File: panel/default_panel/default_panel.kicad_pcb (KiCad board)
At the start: 2 copper layers, 100 x 100 mm, 1 part

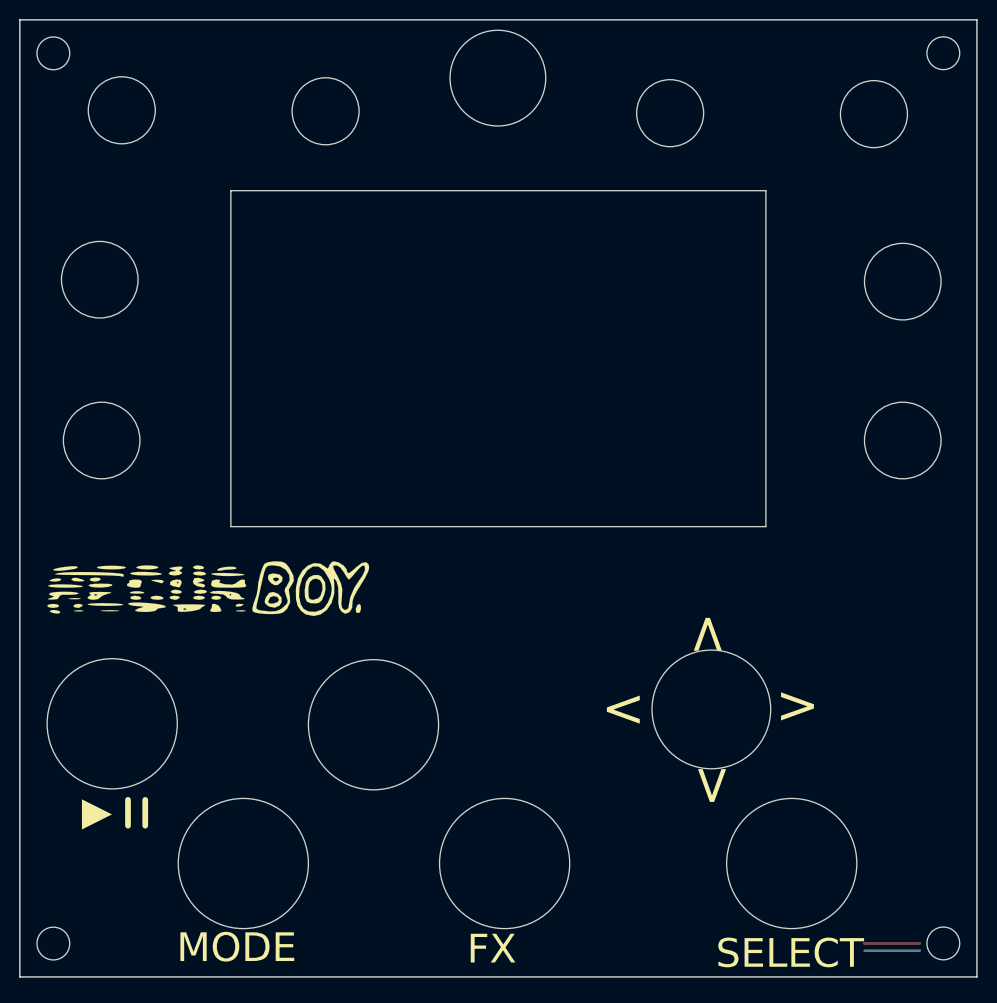
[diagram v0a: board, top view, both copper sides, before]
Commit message: add panel stuff
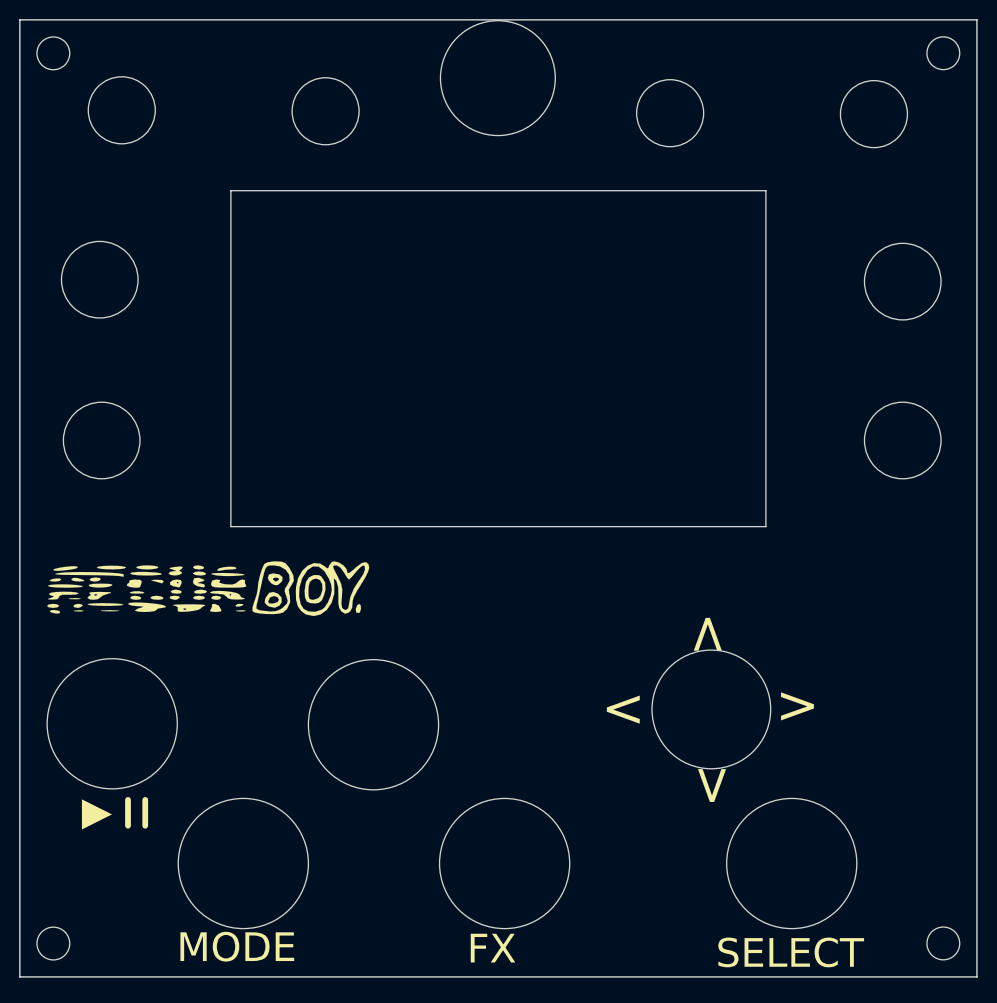
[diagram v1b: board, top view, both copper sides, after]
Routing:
- net (no net): track 11.6 -> 0.00 mm
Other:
- outline, holes or cut-outs redrawn
- board text added: "default_panel mk_iii for recurBOY v0_7_1 cyberboy666 & ichi raramuri"
- board text removed: "cyberboy666 & ichi raramuri recurBOY panel for v0_7_1 mk_ii"
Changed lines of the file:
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@@
       (drillshape 0)
       (scaleselection 1)
-      (outputdirectory "recurBOY_default_panel_v0_7_1_mk_ii")
+      (outputdirectory "recurBOY_default_panel_v0_7_1_mk_iii")
     )
   )
@@
   (gr_line (start 92.95 126.25) (end 92.95 128.95) (layer "F.SilkS") (width 0.6))
   (gr_circle (center 105 132.9) (end 111.8 132.9) (layer "Edge.Cuts") (width 0.1) (fill none))
-  (gr_circle (center 131.596765 50.838475) (end 136.596765 50.838475) (layer "Edge.Cuts") (width 0.1) (fill none))
+  (gr_circle (center 131.596765 50.838475) (end 137.596765 50.838475) (layer "Edge.Cuts") (width 0.1) (fill none))
   (gr_circle (center 91.3 118.3) (end 98.1 118.3) (layer "Edge.Cuts") (width 0.1) (fill none))
   (gr_circle (center 118.6 118.4) (end 125.4 118.4) (layer "Edge.Cuts") (width 0.1) (fill none))
@@
     (effects (font (size 5 5) (thickness 0.5)) (justify mirror))
   )
-  (gr_text "cyberboy666 & ichi raramuri\nrecurBOY panel for v0_7_1 mk_ii" (at 179 131.7 270) (layer "B.SilkS")
+  (gr_text "default_panel mk_iii\nfor recurBOY v0_7_1\ncyberboy666 & ichi raramuri" (at 179 131.7 270) (layer "B.SilkS")
     (effects (font (size 1.2 1.2) (thickness 0.3)) (justify left mirror))
   )
@@
     (effects (font (size 4 4) (thickness 0.8)))
   )
-  (segment (start 169.85 141.25) (end 175.7 141.25) (width 0.25) (layer "F.Cu") (net 0))
-  (segment (start 175.7 142) (end 169.9 142) (width 0.25) (layer "B.Cu") (net 0))
 )
